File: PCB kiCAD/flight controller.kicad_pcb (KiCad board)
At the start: 4 copper layers, 96.5 x 101.6 mm, 28 parts, among them J1 ESC3, J10 RX, J11 V_BATT, J2 ESC4, J3 LED4, J4 LED3, J5 LED1, J6 ESC1, J7 LED2, J8 ESC2, J9 Lidar, U1 YAAJ_BluePill_Part_Like, U2 mpu6050pcb, U3 FTDI, U4 gps, U5 gps, U6 Barometer, U7 mpu6050pcb

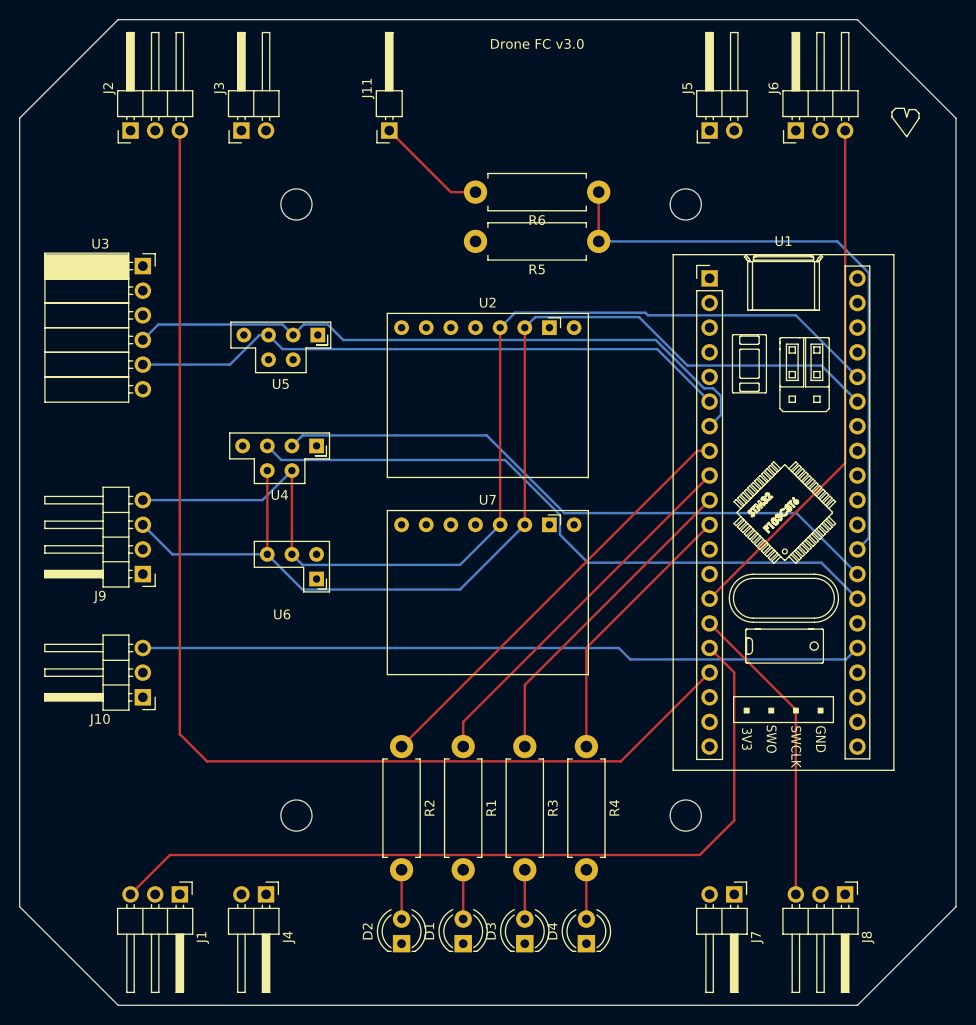
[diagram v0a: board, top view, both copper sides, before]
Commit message: ny pcb
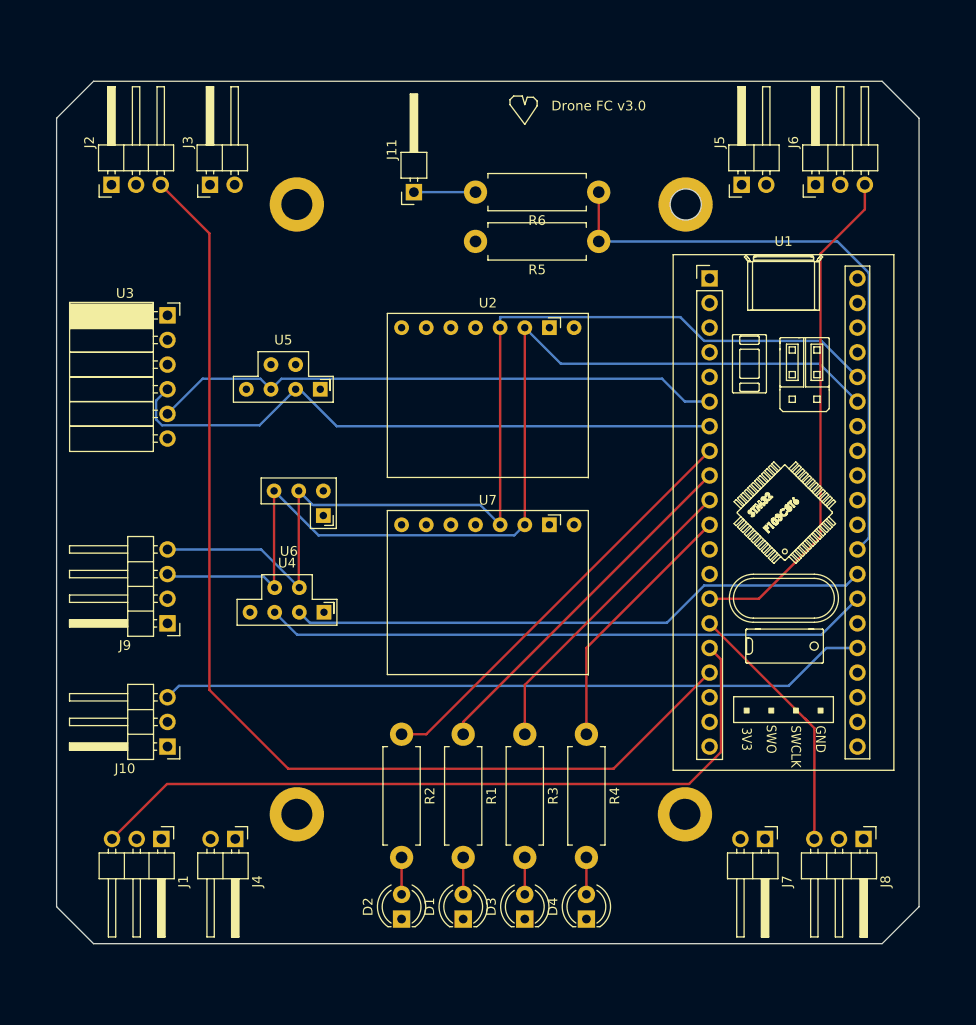
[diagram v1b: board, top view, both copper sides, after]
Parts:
- added REF**: MountingHole_3.2mm_M3_DIN965_Pad, MountingHole:MountingHole_3.2mm_M3_DIN965_Pad, F.Cu at (171.4, 132.7)
- added REF**: MountingHole_3.2mm_M3_DIN965_Pad, MountingHole:MountingHole_3.2mm_M3_DIN965_Pad, F.Cu at (131.4, 132.7)
- added REF**: MountingHole_3.2mm_M3_DIN965_Pad, MountingHole:MountingHole_3.2mm_M3_DIN965_Pad, F.Cu at (171.5, 69.8)
- added REF**: MountingHole_3.2mm_M3_DIN965_Pad, MountingHole:MountingHole_3.2mm_M3_DIN965_Pad, F.Cu at (131.4, 69.8)
- moved U4 17.2 mm to (130.4, 111.9), turned to 0 degrees
- moved J11 6.84 mm to (143.5, 68.6)
- moved U6 6.58 mm to (131.9, 101.8)
- moved J4 6.54 mm to (125.1, 135.3)
- moved J7 6.54 mm to (179.7, 135.3)
- moved J5 6.49 mm to (177.3, 67.8)
- moved J3 6.46 mm to (122.5, 67.8)
- moved J1 6.02 mm to (117.5, 135.3)
- moved J8 6.02 mm to (189.9, 135.3)
- moved J6 5.95 mm to (184.9, 67.8)
- moved J2 5.92 mm to (112.3, 67.8)
- moved J10 5.68 mm to (118.1, 125.7)
- moved J9 5.68 mm to (118.1, 113.0)
- moved U3 5.68 mm to (118.1, 81.3)
- moved U5 5.59 mm to (130.0, 88.9), turned to 0 degrees
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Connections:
- U4 pad 1: Earth -> /5V
- U4 pad 2: /TX2 -> /RX2
- U4 pad 3: /RX2 -> /TX2
- U4 pad 4: /5V -> Earth
- U4 pad 5: /SDA -> /SCL
- U4 pad 6: /SCL -> /SDA
- U5 pad 1: Earth -> /5V
- U5 pad 2: /TX -> /RX
- U5 pad 3: /RX -> /TX
- U5 pad 4: /5V -> Earth
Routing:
- net /ESC4: track 121.8 -> 113.2 mm
- net /ESC3: track 84.2 -> 77.7 mm
- net /RX2: track 68.6 -> 62.6 mm
- net Net-(J11-Pad1): track 11.5 -> 6.35 mm
- net /SCL: track 112.2 -> 107.6 mm
- net /TX2: track 64.7 -> 60.1 mm
- net /ESC2: track 31.6 -> 27.1 mm
- net /TX: track 67.8 -> 64.0 mm
- net /RX: track 62.5 -> 59.3 mm
- net /ESC1: track 54.0 -> 52.3 mm
- net /PPM: track 74.6 -> 73.2 mm
- net Net-(J2-Pad2): track 12.4 -> 11.1 mm
- net /YELLOW_LED: track 33.3 -> 32.0 mm
- net /RED_LED: track 38.5 -> 37.2 mm
- net /BLUE_LED: track 28.1 -> 26.9 mm
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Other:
- board size 96.5 x 101.6 mm -> 88.9 x 88.9 mm
